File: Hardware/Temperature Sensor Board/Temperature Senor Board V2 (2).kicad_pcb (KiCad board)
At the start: 2 copper layers, 41.9 x 26.3 mm, 3 parts

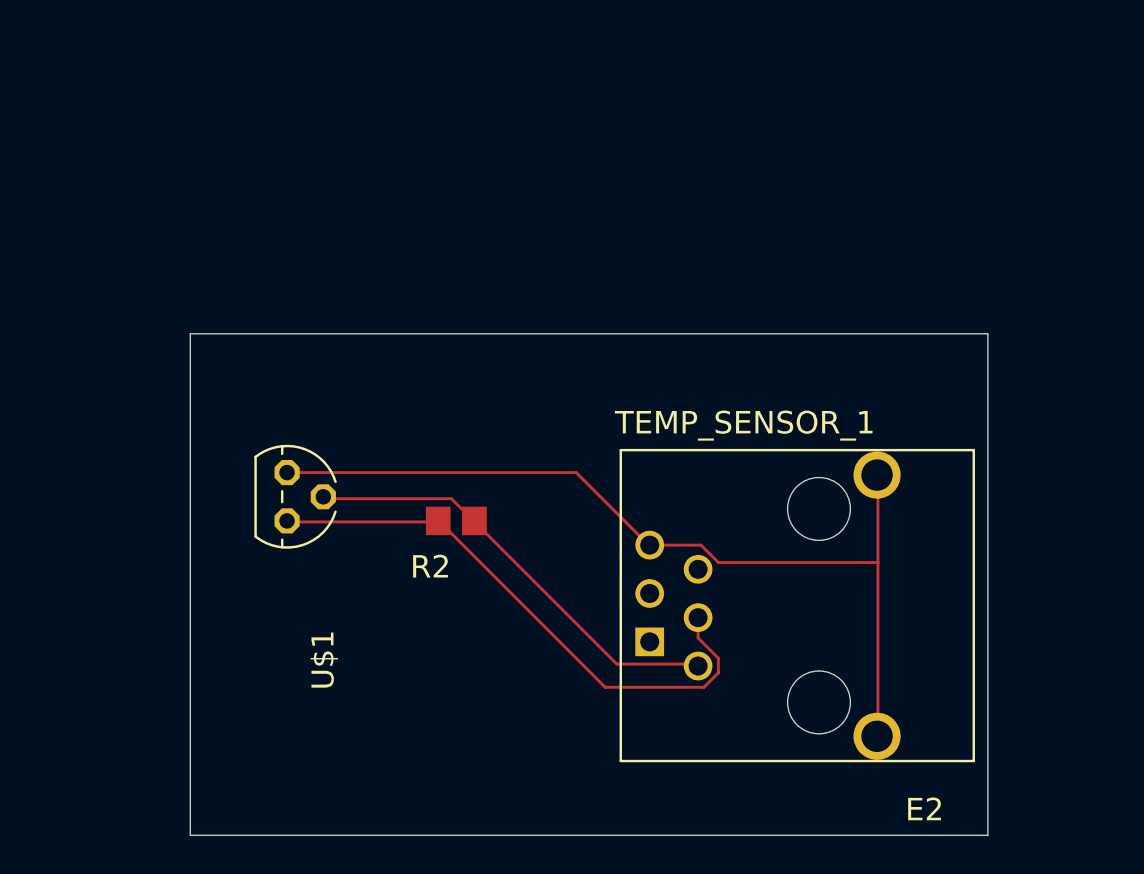
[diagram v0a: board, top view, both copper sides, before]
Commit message: Gerber File  Changed
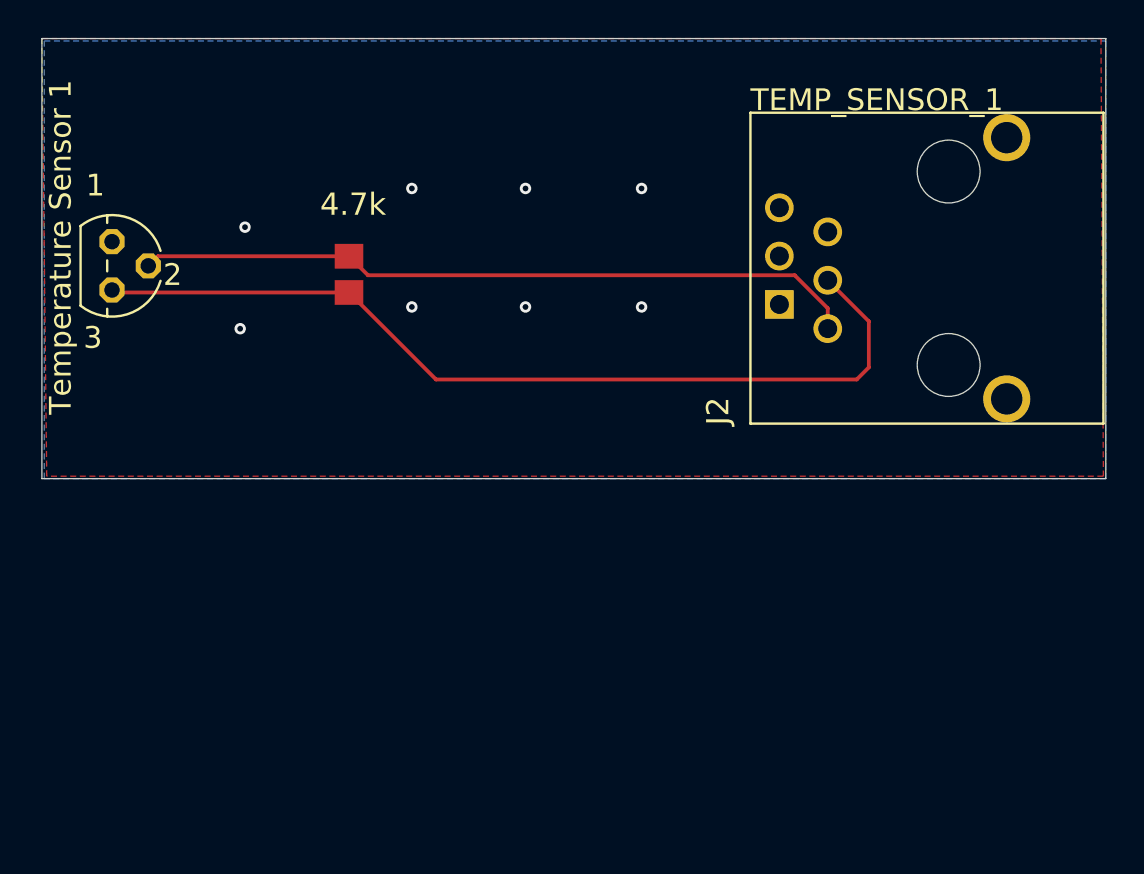
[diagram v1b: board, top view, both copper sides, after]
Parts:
- removed E2: TEMP_SENSOR_1, 1734723-1_RJ11
- removed R2: , R0805
- added 4.7k: R, AutoLoadbankFootprint:R0805, F.Cu at (135.9, 88.7)
- added J2: 6P6C, AutoLoadbankFootprint:1734723-1_RJ11, F.Cu at (161.0, 87.8)
- U$1: value DS18B -> Temperature Sensor 1; footprint TO92 -> AutoLoadbankFootprint:TO92-3
- moved U$1 15.2 mm to (123.4, 88.3)
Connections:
- U$1 pad 1: GND -> /GND
- U$1 pad 2: DQ -> /DQ
- U$1 pad 3: VDD -> /VDD
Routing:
- net /VDD: track 0.00 -> 47.4 mm
- net GND: track 46.8 -> 0.00 mm
- net /DQ: track 0.00 -> 38.1 mm
- net VDD: track 30.0 -> 0.00 mm
- net DQ: track 23.5 -> 0.00 mm
- net /GND: vias 0 -> 8
- added copper zone on B.Cu, net /GND
- added copper zone on F.Cu, net /GND
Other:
- board size 41.9 x 26.3 mm -> 55.9 x 23.1 mm
- board text added: "TEMP_SENSOR_1"
